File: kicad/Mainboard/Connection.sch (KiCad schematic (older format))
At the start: 12 parts, among them J12 GPS_CONN, J13 DBG_CONN, J15 Micro_SD_Card

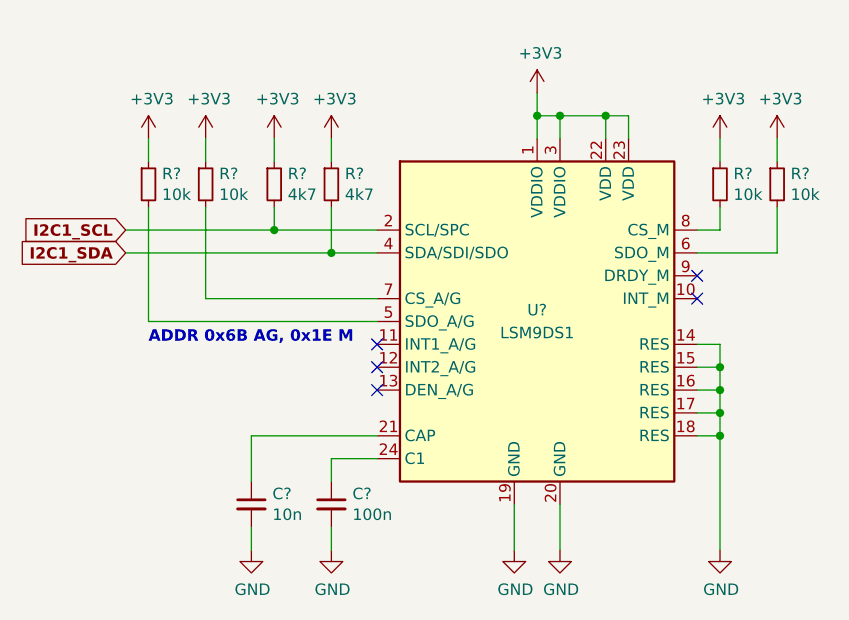
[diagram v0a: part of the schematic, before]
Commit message: Annotated parts
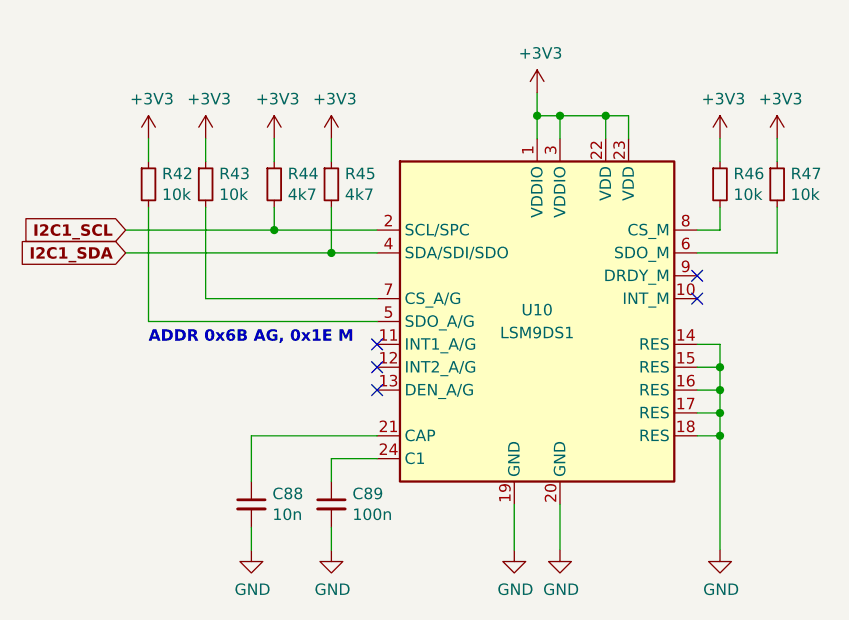
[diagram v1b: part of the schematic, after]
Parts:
- gave numbers to parts that had none: 9
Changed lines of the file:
@@
 TODO: Replace GPS connector
 $Comp
-L Sensor_Motion:LSM9DS1 U?
+L Sensor_Motion:LSM9DS1 U10
 U 1 1 5E067250
 P 7750 3750
-F 0 "U?" H 7750 3800 50  0000 C CNN
+F 0 "U10" H 7750 3800 50  0000 C CNN
 F 1 "LSM9DS1" H 7750 3700 50  0000 C CNN
 F 2 "Package_LGA:LGA-24L_3x3.5mm_P0.43mm" H 9250 4500 50  0001 C CNN
@@
 $EndComp
 $Comp
-L power:+3V3 #PWR?
+L power:+3V3 #PWR0152
 U 1 1 5E06CB2E
 P 7750 2750
-F 0 "#PWR?" H 7750 2600 50  0001 C CNN
+F 0 "#PWR0152" H 7750 2600 50  0001 C CNN
 F 1 "+3V3" H 7765 2923 50  0000 C CNN
 F 2 "" H 7750 2750 50  0001 C CNN
@@
 Connection ~ 8050 2850
 $Comp
-L power:GND #PWR?
+L power:GND #PWR0151
 U 1 1 5E06F5C7
 P 7650 4750
-F 0 "#PWR?" H 7650 4500 50  0001 C CNN
+F 0 "#PWR0151" H 7650 4500 50  0001 C CNN
 F 1 "GND" H 7655 4577 50  0000 C CNN
 F 2 "" H 7650 4750 50  0001 C CNN
@@
 $EndComp
 $Comp
-L power:GND #PWR?
+L power:GND #PWR0153
 U 1 1 5E06FFF0
 P 7850 4750
-F 0 "#PWR?" H 7850 4500 50  0001 C CNN
+F 0 "#PWR0153" H 7850 4500 50  0001 C CNN
 F 1 "GND" H 7855 4577 50  0000 C CNN
 F 2 "" H 7850 4750 50  0001 C CNN
@@
 $EndComp
 $Comp
-L power:GND #PWR?
+L power:GND #PWR0155
 U 1 1 5E070F61
 P 8550 4750
-F 0 "#PWR?" H 8550 4500 50  0001 C CNN
+F 0 "#PWR0155" H 8550 4500 50  0001 C CNN
 F 1 "GND" H 8555 4577 50  0000 C CNN
 F 2 "" H 8550 4750 50  0001 C CNN
@@
 	8550 3950 8550 4050
 $Comp
-L Device:R_Small R?
+L Device:R_Small R45
 U 1 1 5E07451A
 P 6850 3150
-F 0 "R?" H 6909 3196 50  0000 L CNN
+F 0 "R45" H 6909 3196 50  0000 L CNN
 F 1 "4k7" H 6909 3105 50  0000 L CNN
 F 2 "" H 6850 3150 50  0001 C CNN
@@
 $EndComp
 $Comp
-L Device:R_Small R?
+L Device:R_Small R44
 U 1 1 5E075066
 P 6600 3150
-F 0 "R?" H 6659 3196 50  0000 L CNN
+F 0 "R44" H 6659 3196 50  0000 L CNN
 F 1 "4k7" H 6659 3105 50  0000 L CNN
 F 2 "" H 6600 3150 50  0001 C CNN
@@
 Connection ~ 6850 3450
 $Comp
-L power:+3V3 #PWR?
+L power:+3V3 #PWR0149
 U 1 1 5E0788C1
 P 6850 2950
-F 0 "#PWR?" H 6850 2800 50  0001 C CNN
+F 0 "#PWR0149" H 6850 2800 50  0001 C CNN
 F 1 "+3V3" H 6865 3123 50  0000 C CNN
 F 2 "" H 6850 2950 50  0001 C CNN
@@
 $EndComp
 $Comp
-L power:+3V3 #PWR?
+L power:+3V3 #PWR0148
 U 1 1 5E078F90
 P 6600 2950
-F 0 "#PWR?" H 6600 2800 50  0001 C CNN
+F 0 "#PWR0148" H 6600 2800 50  0001 C CNN
 F 1 "+3V3" H 6615 3123 50  0000 C CNN
 F 2 "" H 6600 2950 50  0001 C CNN
@@
 	6850 2950 6850 3050
 $Comp
-L Device:C_Small C?
+L Device:C_Small C89
 U 1 1 5E07AC5C
 P 6850 4550
-F 0 "C?" H 6942 4596 50  0000 L CNN
+F 0 "C89" H 6942 4596 50  0000 L CNN
 F 1 "100n" H 6942 4505 50  0000 L CNN
 F 2 "" H 6850 4550 50  0001 C CNN
@@
 $EndComp
 $Comp
-L Device:C_Small C?
+L Device:C_Small C88
 U 1 1 5E07BBD5
 P 6500 4550
-F 0 "C?" H 6592 4596 50  0000 L CNN
+F 0 "C88" H 6592 4596 50  0000 L CNN
 F 1 "10n" H 6592 4505 50  0000 L CNN
 F 2 "" H 6500 4550 50  0001 C CNN
@@
 	6850 4350 6850 4450
 $Comp
-L power:GND #PWR?
+L power:GND #PWR0150
 U 1 1 5E07DD63
 P 6850 4750
-F 0 "#PWR?" H 6850 4500 50  0001 C CNN
+F 0 "#PWR0150" H 6850 4500 50  0001 C CNN
 F 1 "GND" H 6855 4577 50  0000 C CNN
 F 2 "" H 6850 4750 50  0001 C CNN
@@
 $EndComp
 $Comp
-L power:GND #PWR?
+L power:GND #PWR0147
 U 1 1 5E07E2EE
 P 6500 4750
-F 0 "#PWR?" H 6500 4500 50  0001 C CNN
+F 0 "#PWR0147" H 6500 4500 50  0001 C CNN
 F 1 "GND" H 6505 4577 50  0000 C CNN
 F 2 "" H 6500 4750 50  0001 C CNN
@@
 	8550 4250 8550 4750
 $Comp
-L Device:R_Small R?
+L Device:R_Small R43
 U 1 1 5E085D7F
 P 6300 3150
-F 0 "R?" H 6359 3196 50  0000 L CNN
+F 0 "R43" H 6359 3196 50  0000 L CNN
 F 1 "10k" H 6359 3105 50  0000 L CNN
 F 2 "" H 6300 3150 50  0001 C CNN
@@
 $EndComp
 $Comp
-L Device:R_Small R?
+L Device:R_Small R46
 U 1 1 5E086057
 P 8550 3150
-F 0 "R?" H 8609 3196 50  0000 L CNN
+F 0 "R46" H 8609 3196 50  0000 L CNN
 F 1 "10k" H 8609 3105 50  0000 L CNN
 F 2 "" H 8550 3150 50  0001 C CNN
@@
 	8550 3350 8550 3250
 $Comp
-L power:+3V3 #PWR?
+L power:+3V3 #PWR0146
 U 1 1 5E089278
 P 6300 2950
-F 0 "#PWR?" H 6300 2800 50  0001 C CNN
+F 0 "#PWR0146" H 6300 2800 50  0001 C CNN
 F 1 "+3V3" H 6315 3123 50  0000 C CNN
 F 2 "" H 6300 2950 50  0001 C CNN
@@
 	6300 2950 6300 3050
 $Comp
-L power:+3V3 #PWR?
+L power:+3V3 #PWR0154
 U 1 1 5E08A7A1
 P 8550 2950
-F 0 "#PWR?" H 8550 2800 50  0001 C CNN
+F 0 "#PWR0154" H 8550 2800 50  0001 C CNN
 F 1 "+3V3" H 8565 3123 50  0000 C CNN
 F 2 "" H 8550 2950 50  0001 C CNN
@@
 NoConn ~ 8450 3550
 $Comp
-L Device:R_Small R?
+L Device:R_Small R47
 U 1 1 5E0918A1
 P 8800 3150
-F 0 "R?" H 8859 3196 50  0000 L CNN
+F 0 "R47" H 8859 3196 50  0000 L CNN
 F 1 "10k" H 8859 3105 50  0000 L CNN
 F 2 "" H 8800 3150 50  0001 C CNN
@@
 	8800 3450 8800 3250
 $Comp
-L Device:R_Small R?
+L Device:R_Small R42
 U 1 1 5E092F27
 P 6050 3150
-F 0 "R?" H 6109 3196 50  0000 L CNN
+F 0 "R42" H 6109 3196 50  0000 L CNN
 F 1 "10k" H 6109 3105 50  0000 L CNN
 F 2 "" H 6050 3150 50  0001 C CNN
@@
 	6050 3750 6050 3250
 $Comp
-L power:+3V3 #PWR?
+L power:+3V3 #PWR0145
 U 1 1 5E09497A
 P 6050 2950
-F 0 "#PWR?" H 6050 2800 50  0001 C CNN
+F 0 "#PWR0145" H 6050 2800 50  0001 C CNN
 F 1 "+3V3" H 6065 3123 50  0000 C CNN
 F 2 "" H 6050 2950 50  0001 C CNN
@@
 	6050 2950 6050 3050
 $Comp
-L power:+3V3 #PWR?
+L power:+3V3 #PWR0156
 U 1 1 5E09620D
 P 8800 2950
-F 0 "#PWR?" H 8800 2800 50  0001 C CNN
+F 0 "#PWR0156" H 8800 2800 50  0001 C CNN
 F 1 "+3V3" H 8815 3123 50  0000 C CNN
 F 2 "" H 8800 2950 50  0001 C CNN
